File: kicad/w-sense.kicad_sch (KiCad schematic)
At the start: 40 parts, among them Q1 MMBT3906, SW1 reset, SW2 boot, U1 ESP32-C3FH4, X1 SMD0603-4, Y1 32.768kHz

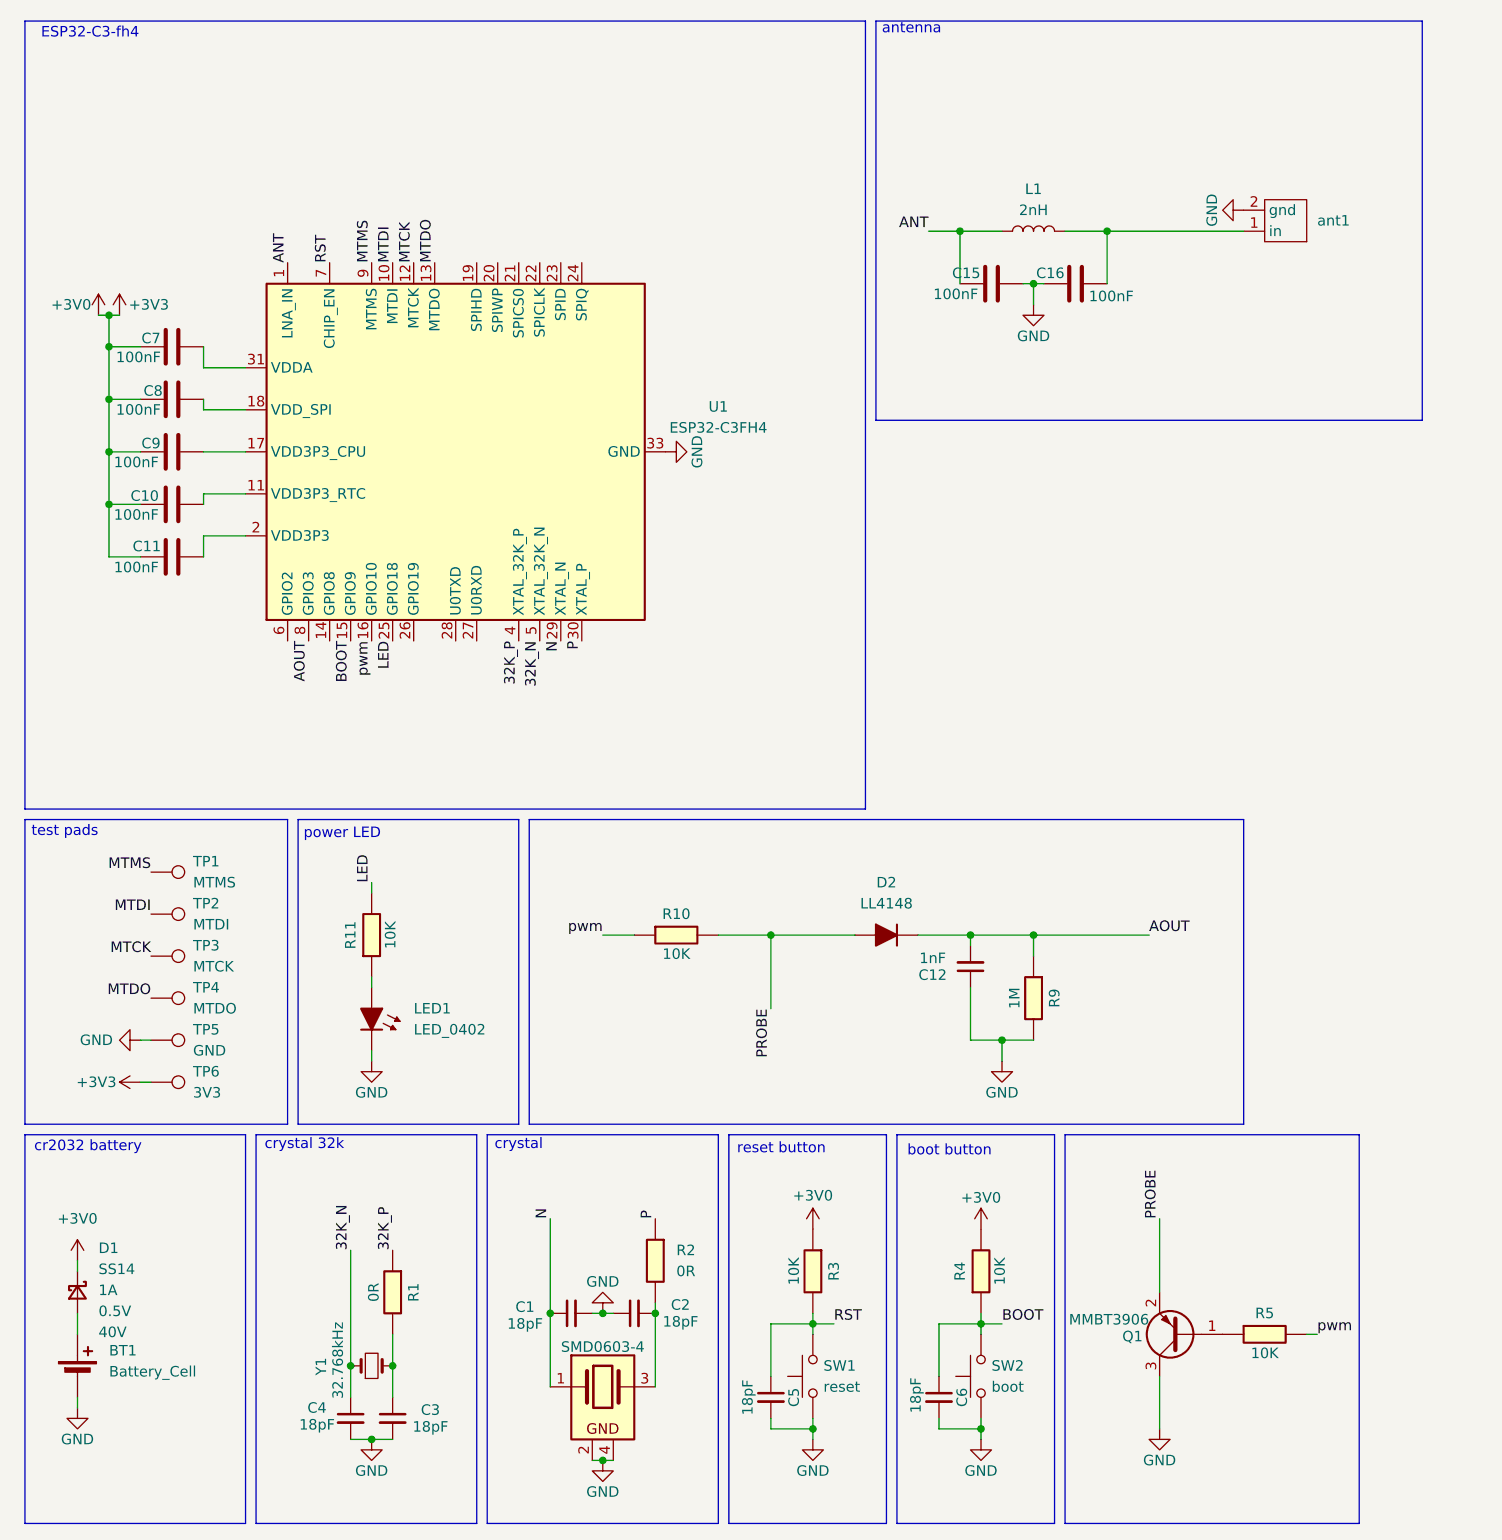
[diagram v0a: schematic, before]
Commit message: finished pcb and schematic
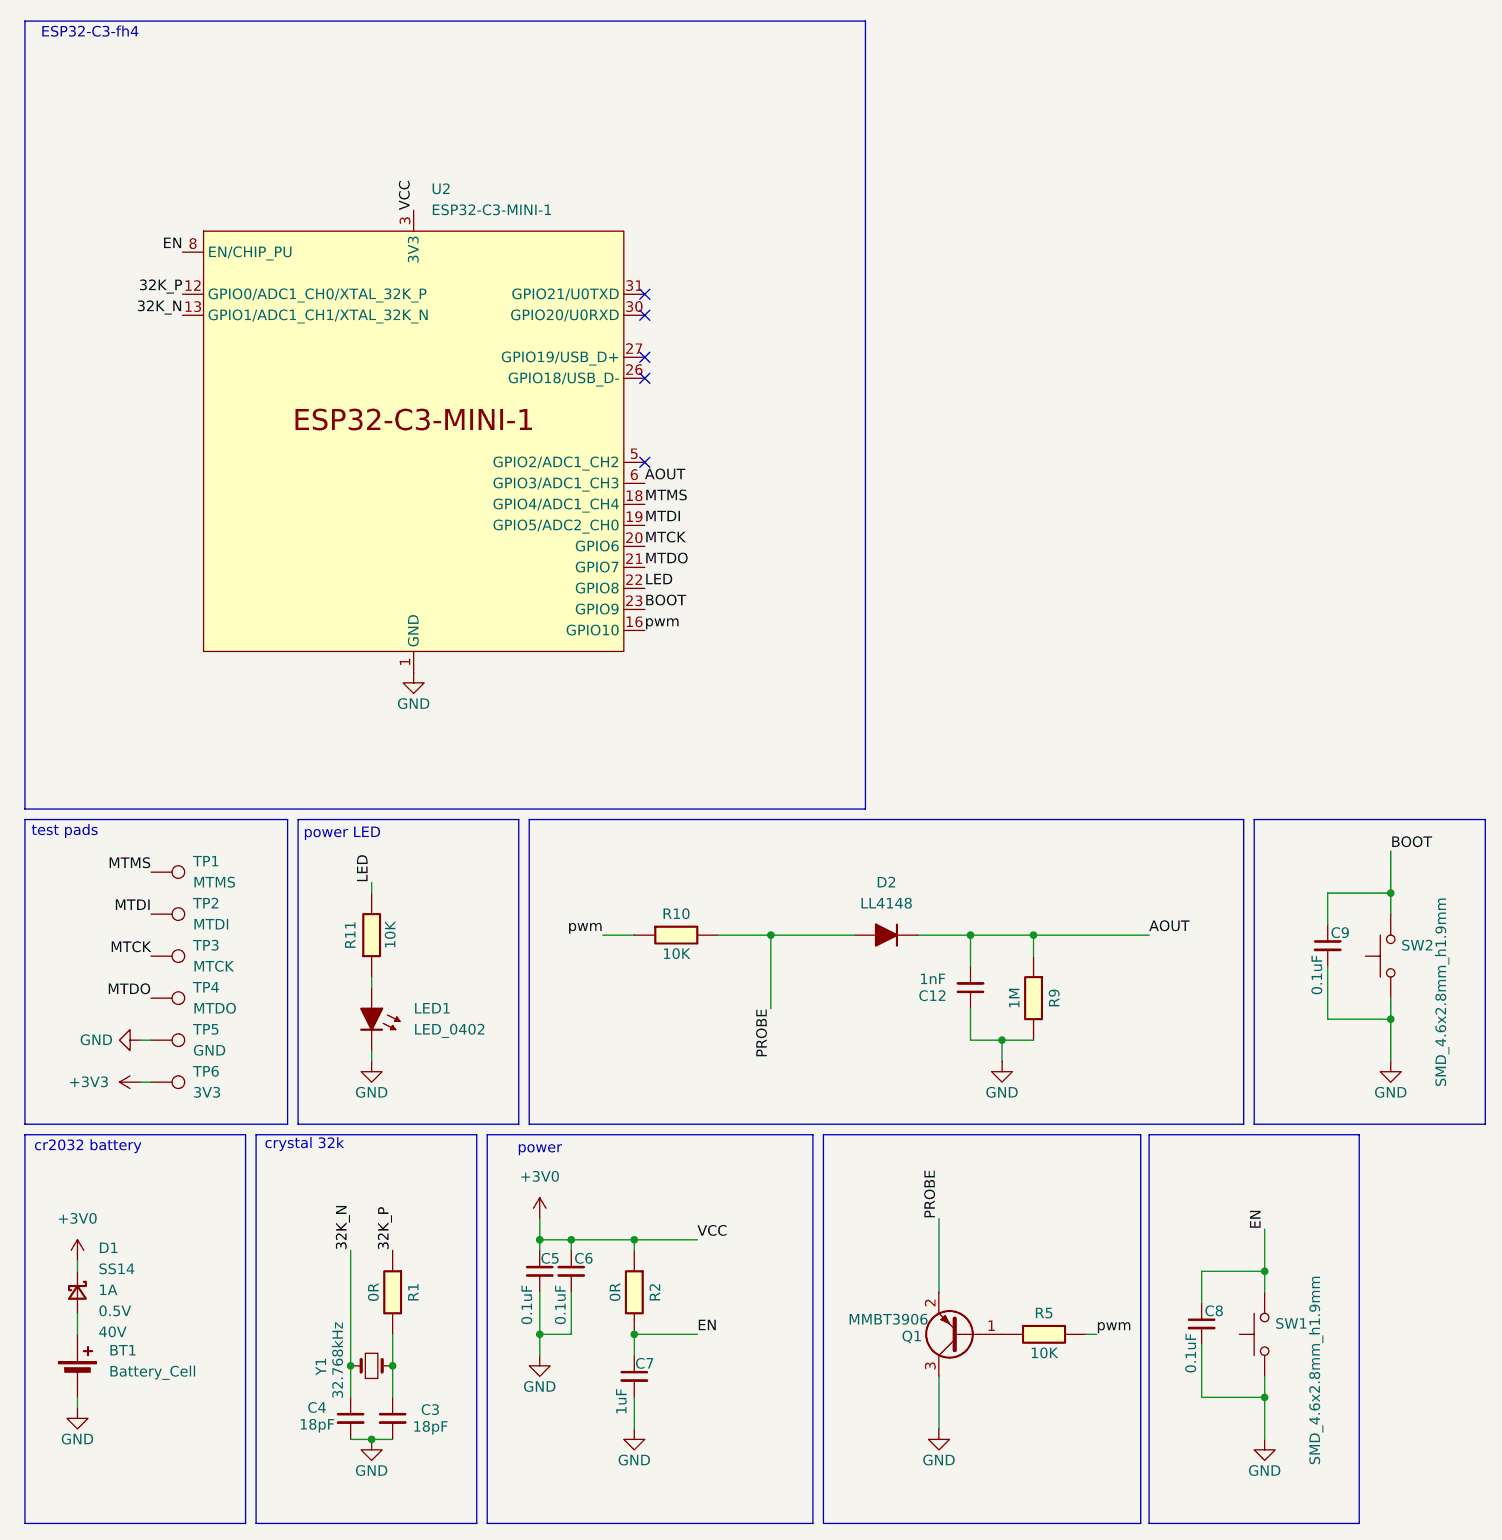
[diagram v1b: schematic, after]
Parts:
- removed C1, C2: 18pF, PCM_SparkFun-Capacitor:C_0603_1608Metric, symbol PCM_SparkFun-Capacitor:18pF_0603_50V_5%
- removed C10, C11, C15, C16, C7, C8, C9: 100nF, Capacitor_SMD:C_0603_1608Metric, symbol Device:C
- removed L1: 2nH, Inductor_SMD:L_0603_1608Metric, symbol Device:L
- removed R3, R4: 10K, PCM_fab:R_0603, symbol PCM_fab:R_0603
- removed SW1: reset, PCM_SparkFun-Switch:Push_SMD_4.2x3.2mm, symbol PCM_SparkFun-Switch:SPST_Push_SMD_6x3.5mm_h2.5mm
- removed SW2: boot, PCM_SparkFun-Switch:Push_SMD_4.2x3.2mm, symbol PCM_SparkFun-Switch:SPST_Push_SMD_6x3.5mm_h2.5mm
- removed U1: ESP32-C3FH4, Package_DFN_QFN:QFN-32-1EP_5x5mm_P0.5mm_EP3.7x3.7mm, symbol MCU_Espressif:ESP32-C3
- removed X1: SMD0603-4, PCM_Crystal_AKL:Crystal_SMD_2520-4Pin_2.5x2.0mm, symbol PCM_Crystal_AKL:SMD0603-4
- removed ant1: (no value), RF_Antenna:Texas_SWRA117D_2.4GHz_Right, symbol rf-antennas:antenna
- added C7: 1uF, Capacitor_SMD:C_0402_1005Metric, symbol PCM_SparkFun-Capacitor:18pF_0603_50V_5%
- added C8, C9: 0.1uF, Capacitor_SMD:C_0402_1005Metric, symbol PCM_SparkFun-Capacitor:18pF_0603_50V_5%
- added SW1, SW2: SMD_4.6x2.8mm_h1.9mm, PCM_SparkFun-Switch:Push_SMD_4.6x2.8mm_h1.9mm, symbol PCM_SparkFun-Switch:SPST_Push_SMD_4.6x2.8mm_h1.9mm
- added U2: ESP32-C3-MINI-1, PCM_Espressif:ESP32-C3-MINI-1, symbol PCM_Espressif:ESP32-C3-MINI-1
- C12, C3, C4: footprint PCM_SparkFun-Capacitor:C_0603_1608Metric -> Capacitor_SMD:C_0402_1005Metric
- C5, C6: value 18pF -> 0.1uF; footprint PCM_SparkFun-Capacitor:C_0603_1608Metric -> Capacitor_SMD:C_0402_1005Metric
- R1, R11, R2, R9: footprint PCM_fab:R_0603 -> Resistor_SMD:R_0402_1005Metric
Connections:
- net P is gone; now on net +3V0: R2.2
- net RST is gone; now on net +3V0: C5.1
- net +3V0: now also C6.1, U2.3 (3V3); no longer TP6.1
- net 32K_N: now also U2.13 (GPIO1/ADC1_CH1/XTAL_32K_N)
- net 32K_P: now also U2.12 (GPIO0/ADC1_CH0/XTAL_32K_P)
- net AOUT: now also U2.6 (GPIO3/ADC1_CH3)
- net BOOT: now also C9.1, SW2.2, U2.23 (GPIO9); no longer C6.1
- net GND: now also C7.2, C8.2, C9.2, SW1.1, SW2.1, U2.1 (GND), U2.11 (GND), U2.14 (GND), U2.2 (GND), U2.36 (GND), U2.37 (GND), U2.38 (GND), U2.39 (GND), U2.40 (GND), U2.41 (GND), U2.42 (GND), U2.43 (GND), U2.44 (GND), U2.45 (GND), U2.46 (GND), U2.47 (GND), U2.48 (GND), U2.49 (GND), U2.50 (GND), U2.51 (GND), U2.52 (GND), U2.53 (GND)
- net LED: now also U2.22 (GPIO8)
- net MTCK: now also U2.20 (GPIO6)
- net MTDI: now also U2.19 (GPIO5/ADC2_CH0)
- net MTDO: now also U2.21 (GPIO7)
- net MTMS: now also U2.18 (GPIO4/ADC1_CH4)
- net pwm: now also U2.16 (GPIO10)
- net EN: now reaches R2.1
- net EN: now also C7.1, C8.1, SW1.2, U2.8 (EN/CHIP_PU)
- new net +3V3: TP6.1
- no-connect marks 0 -> 5
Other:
- note added: "power"
- note removed: "antenna"
- note removed: "boot button"
- note removed: "crystal"
- note removed: "reset button"
- moved on the sheet: C12, Q1, R5
